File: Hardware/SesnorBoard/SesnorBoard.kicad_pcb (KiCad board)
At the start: 2 copper layers, 25 parts, among them U2 CCS811, U3 NC7SVU04P5X, U4 LM324

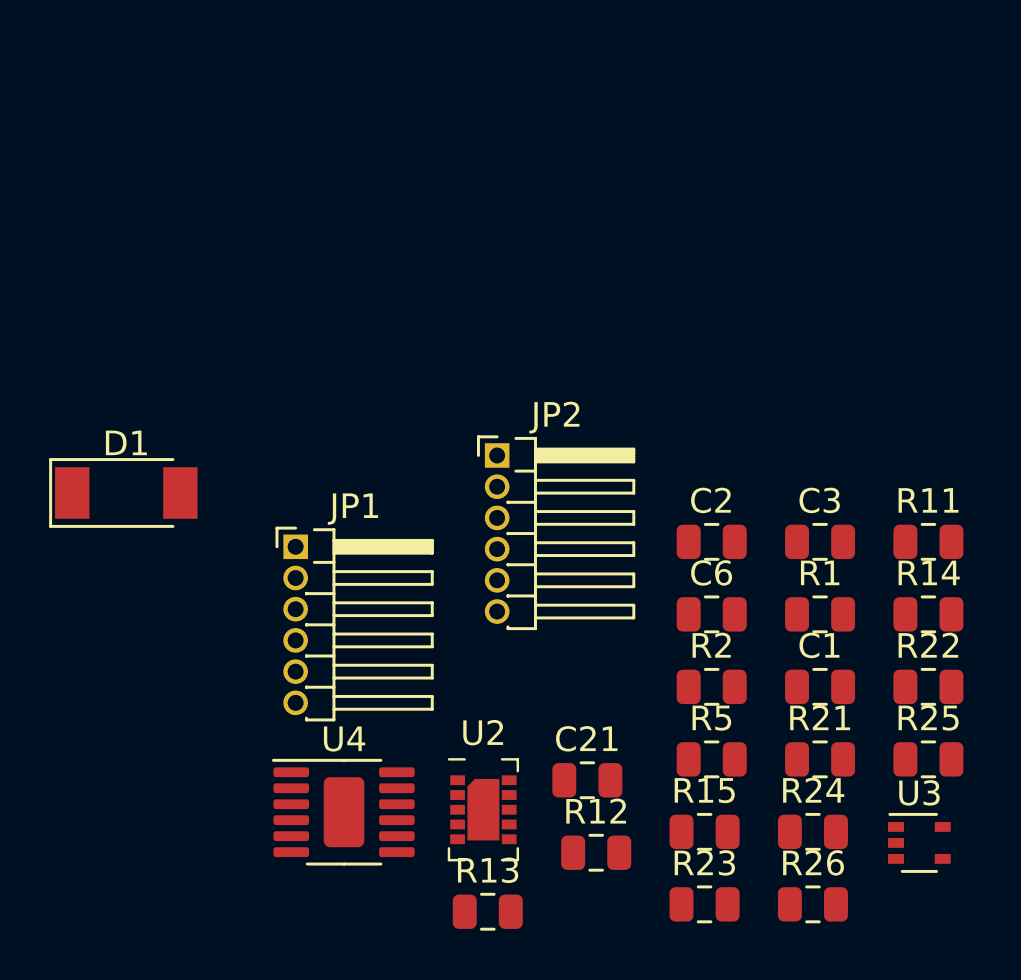
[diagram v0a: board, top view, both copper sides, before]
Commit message: Eerste pcb layouts ensorboard
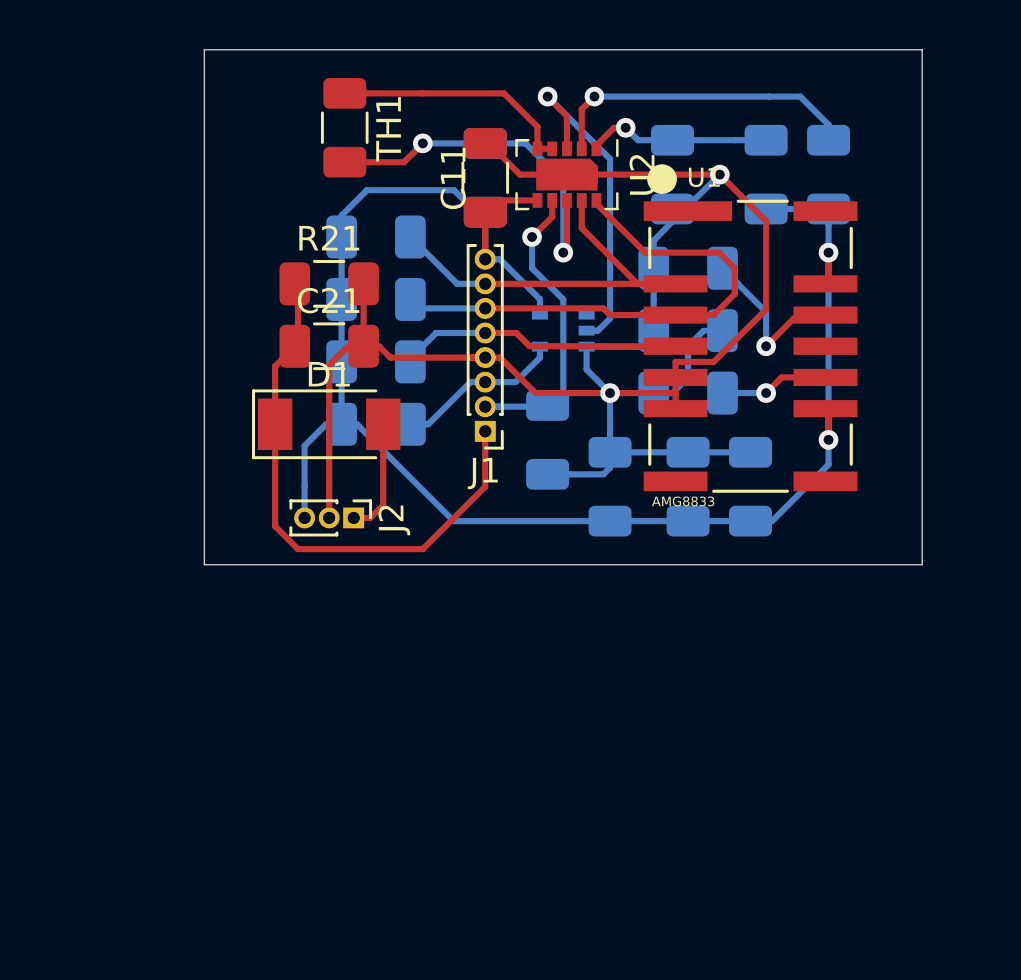
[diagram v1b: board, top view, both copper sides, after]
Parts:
- removed JP1: HEADER POWER & INTERFACE, Connector_PinHeader_1.27mm:PinHeader_1x06_P1.27mm_Horizontal
- removed JP2: HEADER-CONTROL, Connector_PinHeader_1.27mm:PinHeader_1x06_P1.27mm_Horizontal
- removed R22: 1K, Resistor_SMD:R_0805_2012Metric
- removed R23, R24: 10K, Resistor_SMD:R_0805_2012Metric
- removed R25: 100K, Resistor_SMD:R_0805_2012Metric
- removed R26: 100, Resistor_SMD:R_0805_2012Metric
- removed U4: LM324, Package_SO:MSOP-12-1EP_3x4mm_P0.65mm_EP1.65x2.85mm
- added C11: 4.7µF, Capacitor_SMD:C_1206_3216Metric, F.Cu at (68.6, -317.4)
- added J1: Mainboard connection, Connector_PinHeader_1.00mm:PinHeader_1x08_P1.00mm_Vertical, F.Cu at (68.6, -307.1)
- added J2: microphoon connection, Connector_PinHeader_1.00mm:PinHeader_1x03_P1.00mm_Vertical, F.Cu at (63.2, -303.5)
- added R16: 10K, Resistor_SMD:R_1206_3216Metric, B.Cu at (64.1, -307.3)
- added R3: 2k2, Resistor_SMD:R_1206_3216Metric, B.Cu at (64.1, -315.0)
- added R4: 2k2, Resistor_SMD:R_1206_3216Metric, B.Cu at (64.1, -312.4)
- added TH1: 100K, Resistor_SMD:R_1206_3216Metric, F.Cu at (62.9, -319.4)
- added U1: AMG8833, AMG8833_REV-B:AMG8833, F.Cu at (79.4, -310.5)
- C1, C2, C3, C6: footprint Capacitor_SMD:C_0805_2012Metric -> Capacitor_SMD:C_1206_3216Metric; moved to B.Cu
- C21: value 10uF -> 0.1uF; footprint Capacitor_SMD:C_0805_2012Metric -> Capacitor_SMD:C_1206_3216Metric
- D1: value PMEG4050EP -> RB081LAM-20
- R1, R11, R13, R14, R15, R2, R5: footprint Resistor_SMD:R_0805_2012Metric -> Resistor_SMD:R_1206_3216Metric; moved to B.Cu
- R12: value 10K -> 100k; footprint Resistor_SMD:R_0805_2012Metric -> Resistor_SMD:R_1206_3216Metric; moved to B.Cu
- R21: value 2.2K -> 100k; footprint Resistor_SMD:R_0805_2012Metric -> Resistor_SMD:R_1206_3216Metric
- U3: moved to B.Cu
- moved R13 32.1 mm to (80.0, -317.5), turned to 270 degrees
- moved R12 27.8 mm to (68.6, -317.4), turned to 270 degrees
- moved R21 27.8 mm to (62.2, -313.1)
- moved U2 26.1 mm to (71.9, -317.5), turned to 270 degrees
- moved U3 25.4 mm to (71.8, -311.1), turned to 180 degrees
- moved R1 20.8 mm to (64.1, -309.9), turned to 180 degrees
- moved R14 20.7 mm to (76.2, -317.5), turned to 90 degrees
- moved C21 20.5 mm to (62.2, -310.5)
- moved R15 17.2 mm to (71.1, -306.7), turned to 270 degrees
- moved R11 15.5 mm to (82.5, -317.5), turned to 90 degrees
- moved R2 14.5 mm to (76.8, -311.1)
- moved C3 12.4 mm to (76.8, -313.7), turned to 180 degrees
- moved R5 11.2 mm to (79.4, -304.8), turned to 270 degrees
- moved C1 9.76 mm to (76.8, -304.8), turned to 90 degrees
- moved D1 8.72 mm to (62.2, -307.3)
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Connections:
- C21 pad 1: Net-(C21-Pad1) -> /DETECTOR_OUT
- C21 pad 2: Net-(C21-Pad2) -> GND
- D1 pad 1: /DETECTOR-OUT -> /DETECTOR_OUT
- R11 pad 1: +3V3 -> 3.3V
- R12 pad 1: /INT_CSS811 -> Net-(R12-Pad1)
- R12 pad 2: +3V3 -> 3.3V
- R13 pad 2: +3V3 -> 3.3V
- R21 pad 1: Net-(C21-Pad2) -> /DETECTOR_OUT
- R21 pad 2: 3.3V -> GND
- U2 pad 6: +3V3 -> 3.3V
- U2 pad 8: Net-(TH1-Pad1) (its old number) -> Net-(R12-Pad1)
- U3 pad 4: /INT_CSS811 -> /nINT_CCS811
- U3 pad 5: +3V3 -> 3.3V
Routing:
- net GND: track 0.00 -> 72.2 mm, vias 0 -> 2
- net 3.3V: track 0.00 -> 67.2 mm, vias 0 -> 2
- net /DETECTOR_OUT: track 0.00 -> 22.4 mm
- net /SCL: track 0.00 -> 21.7 mm
- net /SDA: track 0.00 -> 18.0 mm
- net Net-(R12-Pad1): track 0.00 -> 14.9 mm, vias 0 -> 2
- net /nINT: track 0.00 -> 14.8 mm, vias 0 -> 1
- net Net-(R11-Pad2): track 0.00 -> 13.0 mm, vias 0 -> 1
- net /nWAKE: track 0.00 -> 12.0 mm, vias 0 -> 1
- net /INT_AMG8833: track 0.00 -> 11.8 mm
- net Net-(TH1-Pad1): track 0.00 -> 9.90 mm
- net Net-(R13-Pad1): track 0.00 -> 8.24 mm, vias 0 -> 1
- net Net-(C3-Pad1): track 0.00 -> 7.48 mm, vias 0 -> 1
- net /nINT_CCS811: track 0.00 -> 6.84 mm
- net Net-(C2-Pad2): track 0.00 -> 5.22 mm
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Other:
- board outline added: 29.2 x 21 mm
